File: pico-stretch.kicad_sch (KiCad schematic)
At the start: 62 parts, among them J1 Conn_01x32_MountingPin, J2 Conn_01x03_Pin, J3 Conn_01x32_MountingPin, U4 Winbond W25Q128JVSIQ, U5 RPI Radio Module 2, U6 ESP-PSRAM32

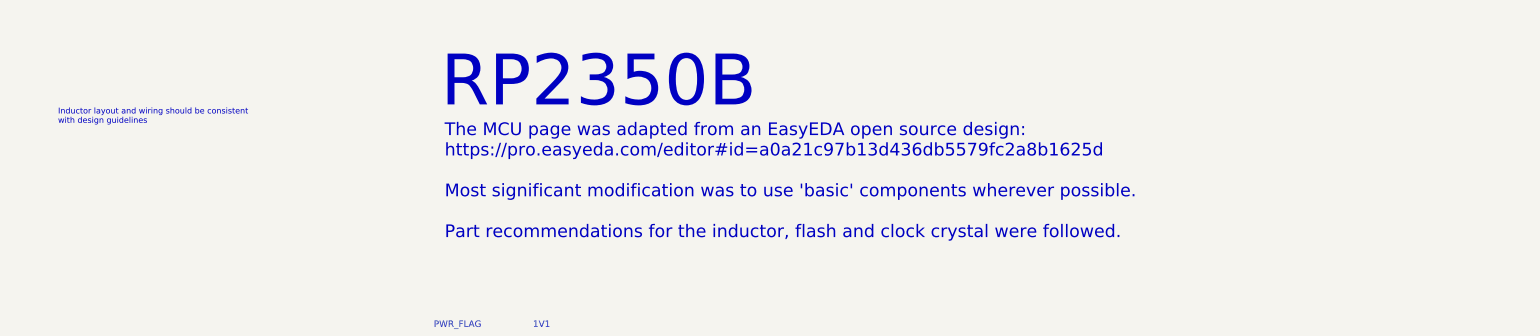
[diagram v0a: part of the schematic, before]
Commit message: Minor text update
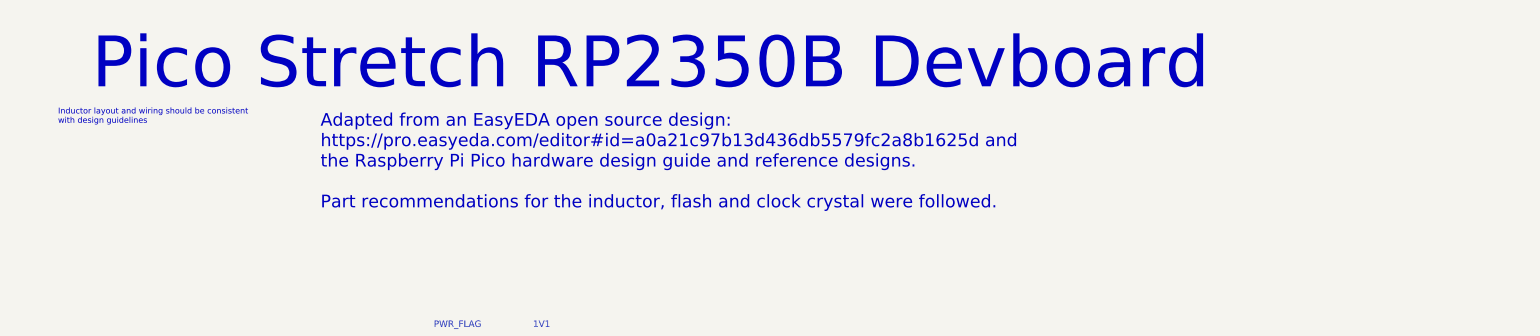
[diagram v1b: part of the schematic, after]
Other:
- note added: "Adapted from an EasyEDA open source design: https://pro.easyeda.com/editor#id=a0a21c97b13d436db5579fc2a8b1625d and the Raspberry Pi Pico hardware design guide and reference designs. Part recommendations for the inductor, flash and clock crystal were followed."
- note added: "Pico Stretch RP2350B Devboard"
- note removed: "RP2350B"
- note removed: "The MCU page was adapted from an EasyEDA open source design: https://pro.easyeda.com/editor#id=a0a21c97b13d436db5579fc2a8b1625d Most significant modification was to use 'basic' components wherever possible. Part recommendations for the inductor, flash and clock crystal were followed."
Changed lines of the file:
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@@
 		)
 	)
-	(text "RP2350B"
+	(text "Pico Stretch RP2350B Devboard"
 		(exclude_from_sim no)
-		(at 126.238 32.004 0)
+		(at 57.658 28.448 0)
 		(effects
 			(font
@@
 		)
 	)
-	(text "The MCU page was adapted from an EasyEDA open source design:\nhttps://pro.easyeda.com/editor#id=a0a21c97b13d436db5579fc2a8b1625d\n\nMost significant modification was to use 'basic' components wherever possible.\n\nPart recommendations for the inductor, flash and clock crystal were followed."
+	(text "Adapted from an EasyEDA open source design:\nhttps://pro.easyeda.com/editor#id=a0a21c97b13d436db5579fc2a8b1625d and\nthe Raspberry Pi Pico hardware design guide and reference designs.\n\nPart recommendations for the inductor, flash and clock crystal were followed."
 		(exclude_from_sim no)
-		(at 127 57.15 0)
+		(at 102.616 51.308 0)
 		(effects
 			(font
